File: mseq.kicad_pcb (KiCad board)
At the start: 2 copper layers, 135.3 x 78.4 mm, 93 parts, among them J1 Screen_I2C, J3 Conn_ARM_JTAG_SWD_10, SW1 RESET, SW2 ON/OFF, SW3 MS/SLAVE, SW4 BOOT, U1 SN74HCT125DR, U2 H11L1M, U3 AMS1117-3.3, U4 STM32F413CHUx, U5 CP2102N-Axx-xQFN20, U6 H11L1M, U7 W25Q16JVSS, U8 MB85RS256B, Y1 32.768kHz ±20ppm 6pF, Y2 25 MHz ±20ppm 18pF

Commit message: chaged the pin name
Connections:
- net /B6 renamed /SCL
- net /B7 renamed /SDA

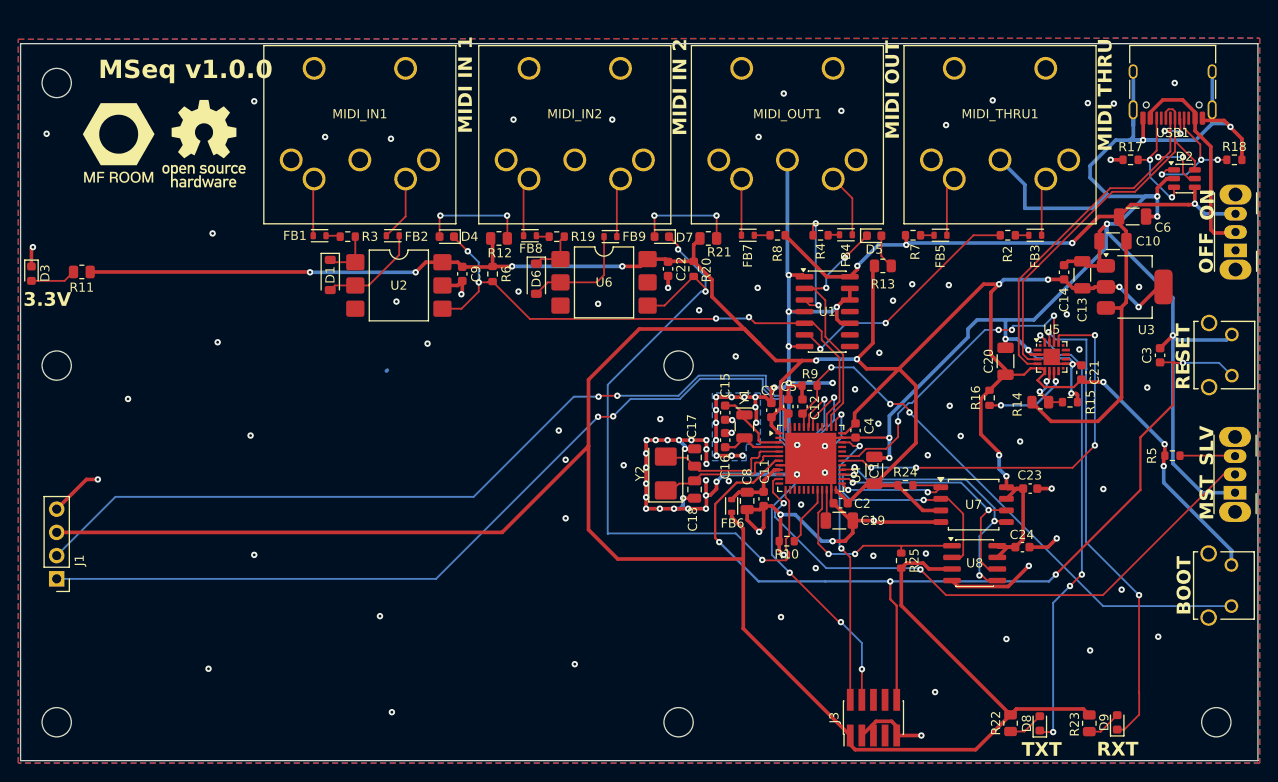
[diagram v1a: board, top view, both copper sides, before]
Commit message: updated
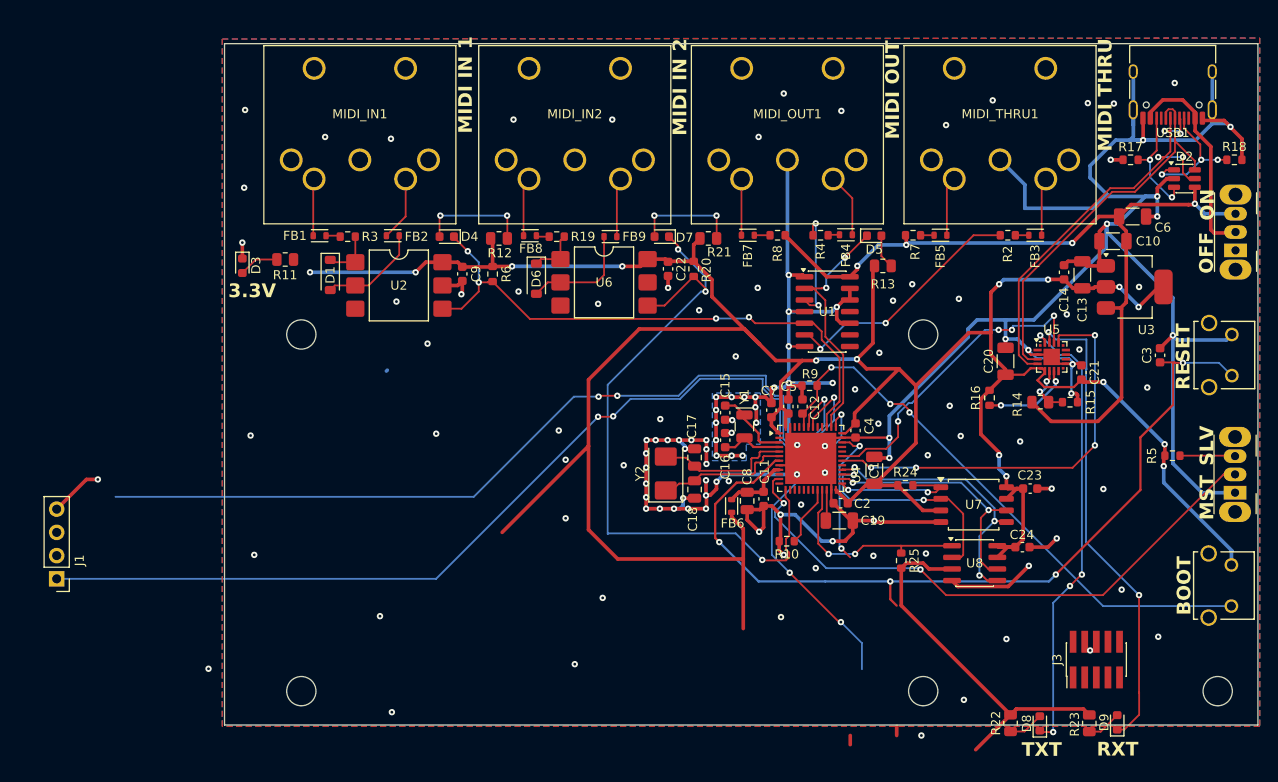
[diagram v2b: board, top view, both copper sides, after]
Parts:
- removed the REF** at (18.2, 52.5)
- moved REF** 27.0 mm to (45.0, 80.0)
- moved REF** 27.0 mm to (45.0, 119.0)
- moved REF** 27.0 mm to (113.0, 80.0)
- moved REF** 27.0 mm to (113.0, 119.0)
- moved J3 25.2 mm to (131.9, 115.5)
- moved D3 23.1 mm to (38.5, 72.5)
- moved R11 22.3 mm to (43.2, 71.8)
- moved REF** 3.40 mm to (145.2, 119.0)
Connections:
- J1 pad 1: /SCL -> GND
- J1 pad 2: /SDA -> +3.3V
- J1 pad 3: +3.3V -> /SCL
- J1 pad 4: GND -> /SDA
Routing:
- net +3.3V: track 486.3 -> 378.9 mm
- net /SWDIO: track 31.2 -> 15.6 mm
- net GND: track 428.5 -> 414.9 mm, vias 134 -> 132
- net /NRST: track 102.6 -> 92.3 mm
- net /SWCLOCK: track 40.2 -> 36.8 mm, vias 4 -> 3
- net /SDA: track 106.7 -> 103.4 mm, vias 3 -> 4
- net Net-(D3-A): track 5.00 -> 4.39 mm
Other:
- board size 135.3 x 78.4 mm -> 113 x 74.5 mm
